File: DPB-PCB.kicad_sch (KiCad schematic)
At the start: 2 parts, among them J1 USB-C, U1 ESP32-S3-WROOM-1-N4R2

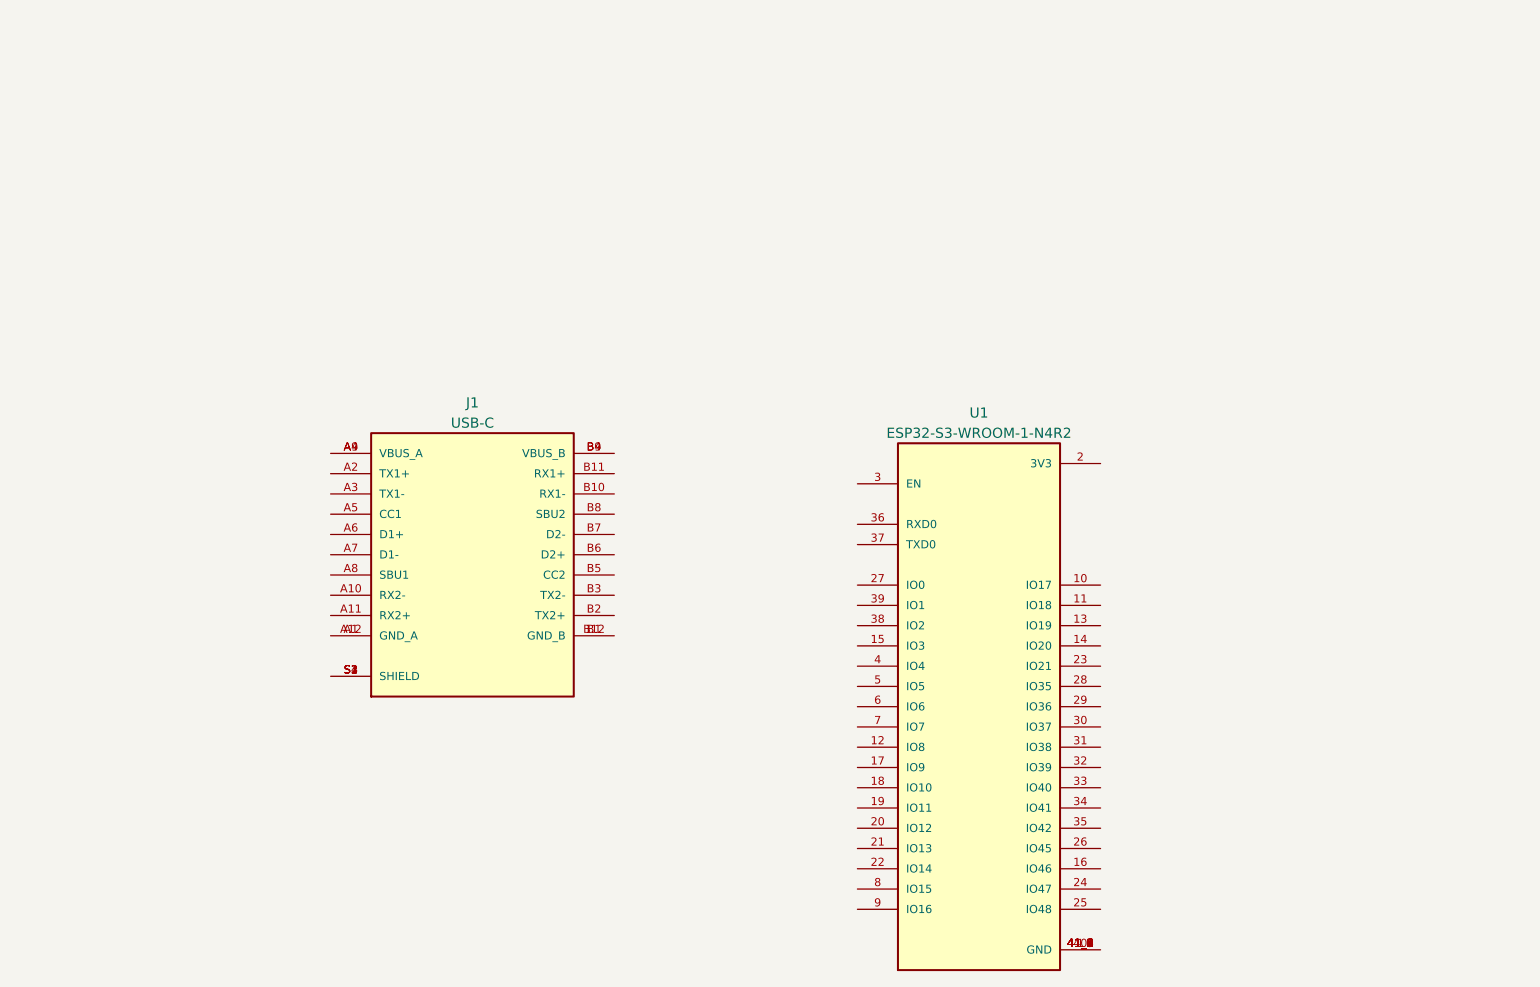
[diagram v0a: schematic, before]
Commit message: up
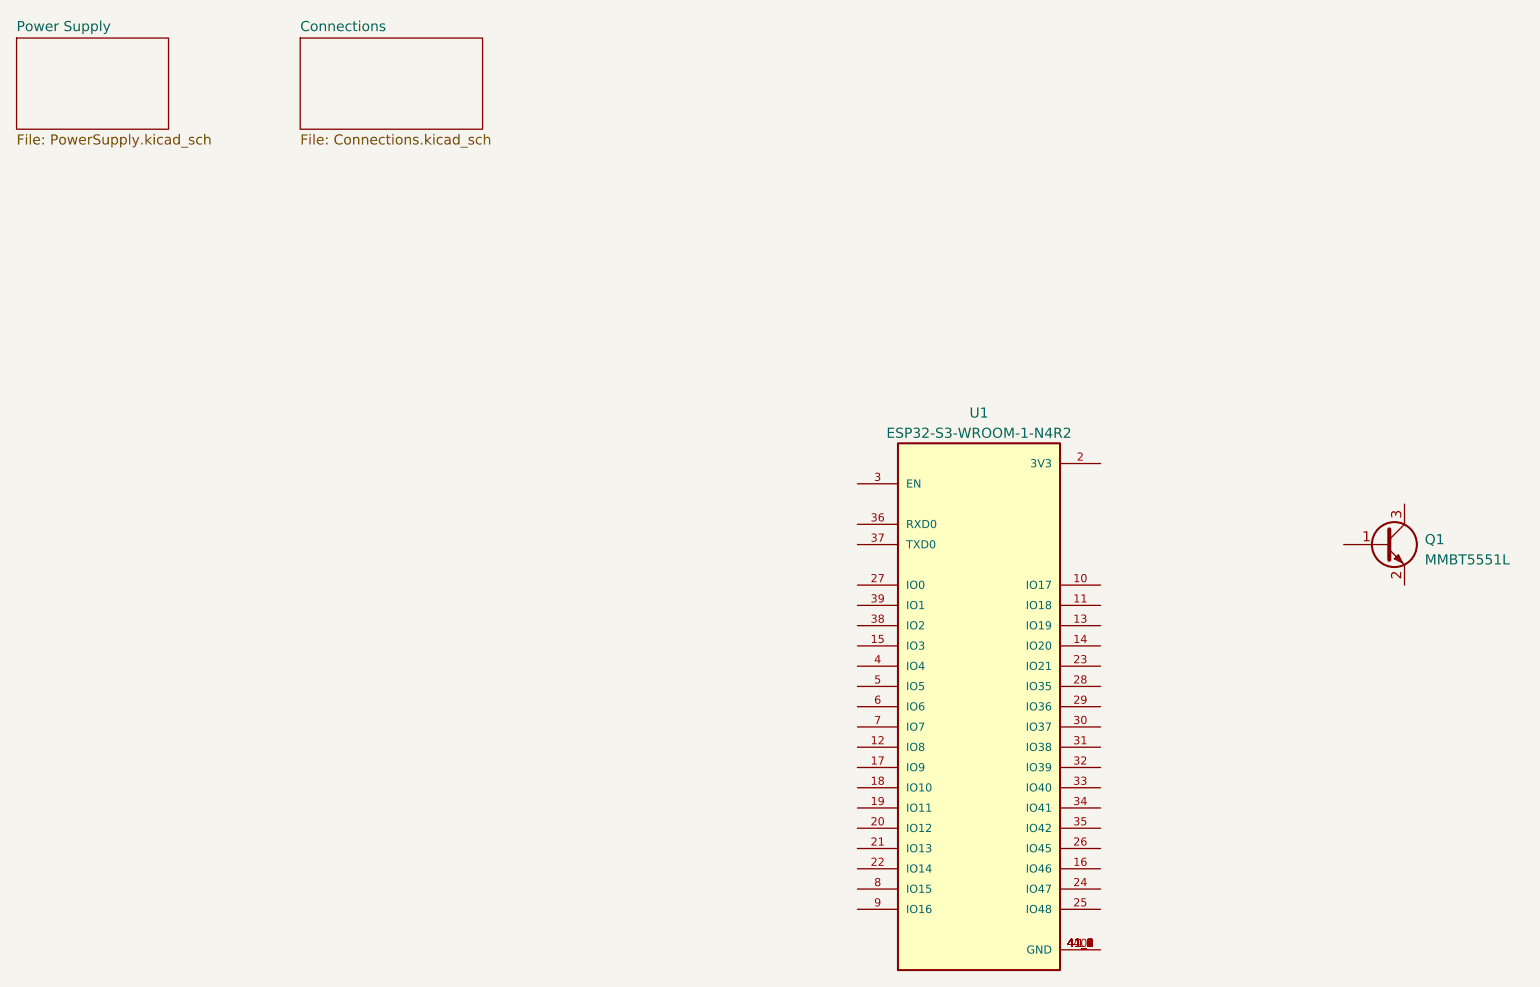
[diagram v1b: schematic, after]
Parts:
- removed J1: USB-C, Library:MOLEX_USB_TYPE_C, symbol MOLEX_USB_TYPE_C:105450-0101
- added Q1: MMBT5551L, Package_TO_SOT_SMD:SOT-23, symbol Transistor_BJT:MMBT5551L
- U1: LCSC (none) -> C2913204; MANUFACTURER Espressif -> (none); MAXIMUM_PACKAGE_HEIGHT 3.25mm -> (none); PARTREV v1.0 -> (none); STANDARD Manufacturer Recommendations -> (none)
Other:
- added sheet Connections (Connections.kicad_sch)
- added sheet Power Supply (PowerSupply.kicad_sch)
- company: (none) -> V2
- title: (none) -> Dynamic propeller balancer
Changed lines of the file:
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@@
 (kicad_sch (version 20230121) (generator eeschema)
   (paper "A4")
-  (symbol (lib_id "MOLEX_USB_TYPE_C:105450-0101") (at 74.93 82.55 0) (unit 1)
-    (in_bom yes) (on_board yes) (dnp no) (fields_autoplaced)
-    (property "Reference" "J1" (at 74.93 63.5 0)
-      (effects (font (size 1.27 1.27)))
-    )
-    (property "Value" "USB-C" (at 74.93 66.04 0)
-      (effects (font (size 1.27 1.27)))
-    )
-    (property "Footprint" "Library:MOLEX_USB_TYPE_C" (at 74.93 82.55 0)
-      (effects (font (size 1.27 1.27)) (justify bottom) hide)
-    )
-    (property "Datasheet" "" (at 74.93 82.55 0)
-      (effects (font (size 1.27 1.27)) hide)
-    )
-    (property "STANDARD" "Manufacturer Recommendations" (at 74.93 82.55 0)
-      (effects (font (size 1.27 1.27)) (justify bottom) hide)
-    )
-    (property "PARTREV" "A7" (at 74.93 82.55 0)
-      (effects (font (size 1.27 1.27)) (justify bottom) hide)
-    )
-    (property "MANUFACTURER" "Molex" (at 74.93 82.55 0)
-      (effects (font (size 1.27 1.27)) (justify bottom) hide)
-    )
-    (property "MAXIMUM_PACKAGE_HEIGHT" "3.24mm" (at 74.93 82.55 0)
-      (effects (font (size 1.27 1.27)) (justify bottom) hide)
-    )
-    (pin "A1")
-    (pin "A10")
-    (pin "A11")
-    (pin "A12")
-    (pin "A2")
-    (pin "A3")
-    (pin "A4")
-    (pin "A5")
-    (pin "A6")
-    (pin "A7")
-    (pin "A8")
-    (pin "A9")
-    (pin "B1")
-    (pin "B10")
-    (pin "B11")
-    (pin "B12")
-    (pin "B2")
-    (pin "B3")
-    (pin "B4")
-    (pin "B5")
-    (pin "B6")
-    (pin "B7")
-    (pin "B8")
-    (pin "B9")
-    (pin "S1")
-    (pin "S2")
-    (pin "S3")
-    (pin "S4")
-    (instances
-      (project "DPB-PCB"
-        (path "/0a09ce58-c923-4e96-b56b-0b86aca559ed"
-          (reference "J1") (unit 1)
-        )
-      )
-    )
+  (title_block
+    (title "Dynamic propeller balancer")
+    (date "2023-02-27")
+    (rev "1")
+    (company "V2")
   )
   (symbol (lib_id "ESP32-S3-WROOM-1-N4R2:ESP32-S3-WROOM-1-N4R2") (at 138.43 101.6 0) (unit 1)
@@
       (effects (font (size 1.27 1.27)) hide)
     )
-    (property "PARTREV" "v1.0" (at 138.43 101.6 0)
-      (effects (font (size 1.27 1.27)) (justify bottom) hide)
-    )
-    (property "MANUFACTURER" "Espressif" (at 138.43 101.6 0)
-      (effects (font (size 1.27 1.27)) (justify bottom) hide)
-    )
-    (property "MAXIMUM_PACKAGE_HEIGHT" "3.25mm" (at 138.43 101.6 0)
-      (effects (font (size 1.27 1.27)) (justify bottom) hide)
-    )
-    (property "STANDARD" "Manufacturer Recommendations" (at 138.43 101.6 0)
-      (effects (font (size 1.27 1.27)) (justify bottom) hide)
+    (property "LCSC" "C2913204" (at 138.43 101.6 0)
+      (effects (font (size 1.27 1.27)) hide)
     )
     (pin "1")
@@
       )
     )
+  )
+  (symbol (lib_id "Transistor_BJT:MMBT5551L") (at 189.23 81.28 0) (unit 1)
+    (in_bom yes) (on_board yes) (dnp no) (fields_autoplaced)
+    (property "Reference" "Q1" (at 194.31 80.645 0)
+      (effects (font (size 1.27 1.27)) (justify left))
+    )
+    (property "Value" "MMBT5551L" (at 194.31 83.185 0)
+      (effects (font (size 1.27 1.27)) (justify left))
+    )
+    (property "Footprint" "Package_TO_SOT_SMD:SOT-23" (at 194.31 83.185 0)
+      (effects (font (size 1.27 1.27) italic) (justify left) hide)
+    )
+    (property "Datasheet" "www.onsemi.com/pub/Collateral/MMBT5550LT1-D.PDF" (at 189.23 81.28 0)
+      (effects (font (size 1.27 1.27)) (justify left) hide)
+    )
+    (property "LCSC" "" (at 189.23 81.28 0)
+      (effects (font (size 1.27 1.27)) hide)
+    )
+    (pin "1")
+    (pin "2")
+    (pin "3")
+    (instances
+      (project "DPB-PCB"
+        (path "/0a09ce58-c923-4e96-b56b-0b86aca559ed"
+          (reference "Q1") (unit 1)
+        )
+      )
+    )
+  )
+  (sheet (at 17.78 17.78) (size 19.05 11.43) (fields_autoplaced)
+    (stroke (width 0.1524) (type solid))
+    (fill (color 0 0 0 0.0000))
+    (property "Sheetname" "Power Supply" (at 17.78 17.0684 0)
+      (effects (font (size 1.27 1.27)) (justify left bottom))
+    )
+    (property "Sheetfile" "PowerSupply.kicad_sch" (at 17.78 29.7946 0)
+      (effects (font (size 1.27 1.27)) (justify left top))
+    )
+    (instances
+      (project "DPB-PCB"
+        (path "/0a09ce58-c923-4e96-b56b-0b86aca559ed" (page "2"))
+      )
+    )
+  )
+  (sheet (at 53.34 17.78) (size 22.86 11.43) (fields_autoplaced)
+    (stroke (width 0.1524) (type solid))
+    (fill (color 0 0 0 0.0000))
+    (property "Sheetname" "Connections" (at 53.34 17.0684 0)
+      (effects (font (size 1.27 1.27)) (justify left bottom))
+    )
+    (property "Sheetfile" "Connections.kicad_sch" (at 53.34 29.7946 0)
+      (effects (font (size 1.27 1.27)) (justify left top))
+    )
+    (instances
+      (project "DPB-PCB"
+        (path "/0a09ce58-c923-4e96-b56b-0b86aca559ed" (page "3"))
+      )
+    )
